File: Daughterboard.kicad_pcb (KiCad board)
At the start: 4 copper layers, 60 parts, among them U1 SI8271GB-IS, U2 SI8271GB-IS, U3 GS61004B, U4 IES0105S09, U5 GS61004B, U6 IES0105S09

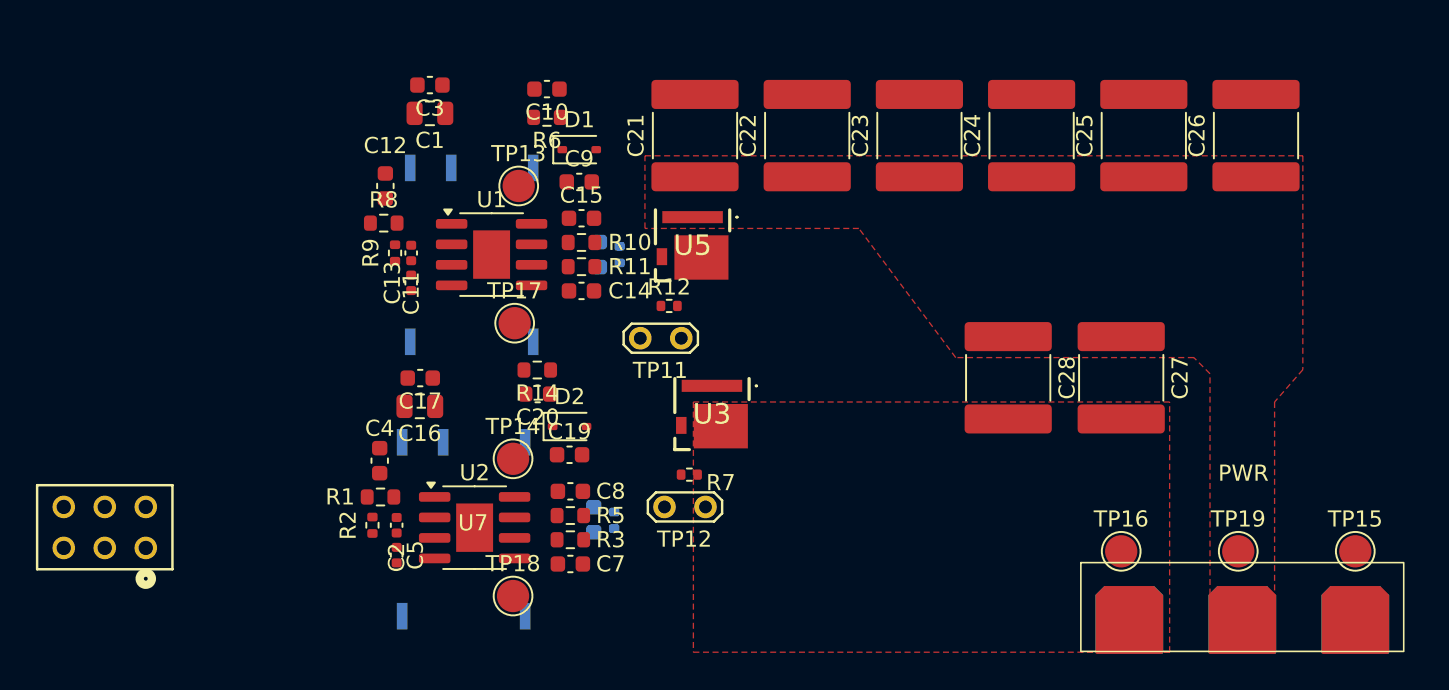
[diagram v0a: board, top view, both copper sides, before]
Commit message: initial version for commenting
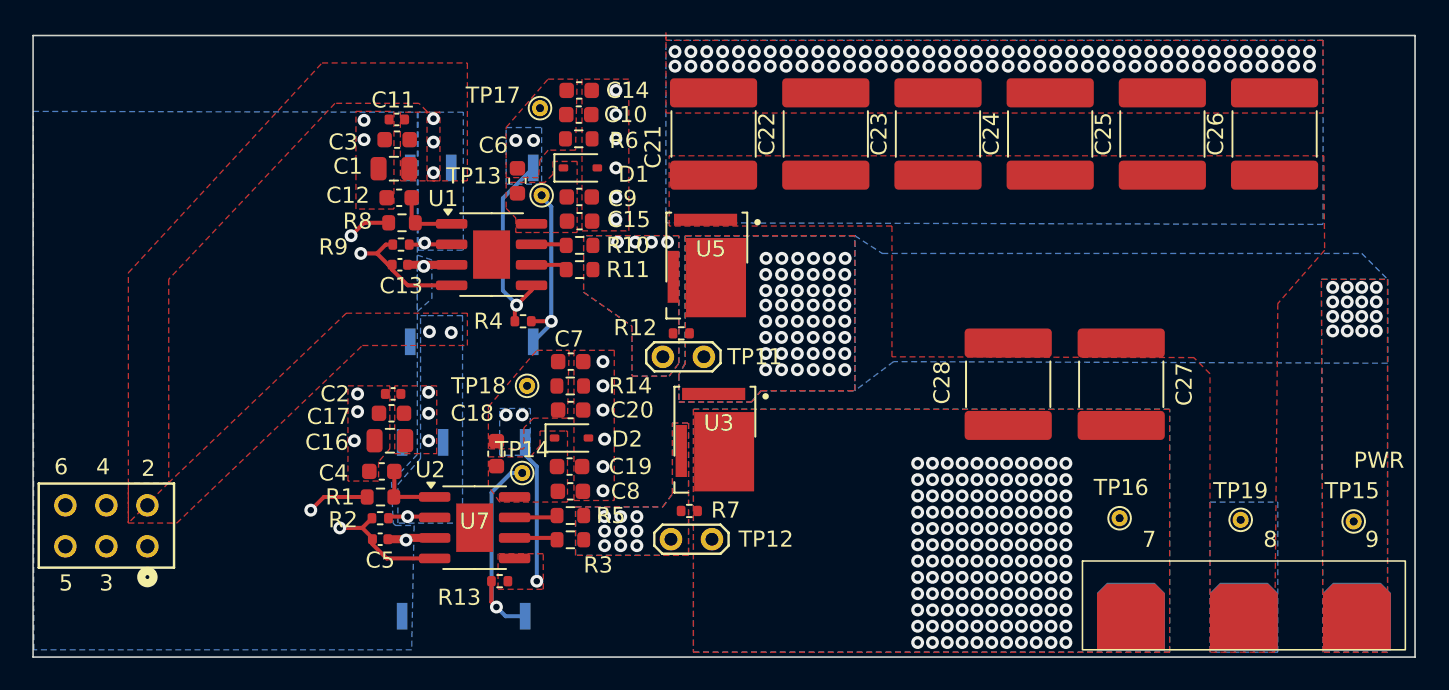
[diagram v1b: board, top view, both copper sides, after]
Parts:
- C18, C6, R13, R4: moved to F.Cu
- TP13, TP14, TP15, TP16, TP17, TP18, TP19: footprint TestPoint:TestPoint_Pad_D2.0mm -> TestPoint:TestPoint_THTPad_D1.0mm_Drill0.5mm
- U3, U5: footprint GS61004B:GS61004B -> GS61004B:GS6XXX4B
- moved TP17 13.4 mm to (110.5, 93.8)
- moved TP18 13.0 mm to (109.7, 111.0)
- moved C7 12.5 mm to (112.4, 109.5)
- moved C14 12.4 mm to (112.9, 92.7)
- moved C11 8.32 mm to (101.6, 94.5), turned to 180 degrees
- moved C2 8.14 mm to (101.4, 111.5), turned to 180 degrees
- moved R13 8.03 mm to (108.0, 123.1), turned to 0 degrees
- moved C18 7.29 mm to (107.8, 115.2)
- moved R4 7.27 mm to (109.5, 107.0), turned to 180 degrees
- moved C6 6.83 mm to (109.1, 98.3)
- moved C1 4.09 mm to (101.5, 97.5)
- moved C3 3.94 mm to (101.7, 95.8)
- moved C16 2.82 mm to (101.2, 114.4)
- moved C17 2.81 mm to (101.3, 112.7)
- moved C10 2.53 mm to (112.9, 94.2)
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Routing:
- net ENABLEH: track 0.00 -> 30.1 mm, vias 0 -> 1
- net PWMH: track 0.00 -> 29.4 mm, vias 0 -> 1
- net PWML: track 0.00 -> 20.8 mm, vias 0 -> 1
- net ENABLEL: track 0.00 -> 20.1 mm, vias 0 -> 1
- net VDDL: track 0.00 -> 13.4 mm, vias 0 -> 1
- net VEEH: track 0.00 -> 12.3 mm, vias 0 -> 3
- net VDDH: track 0.00 -> 11.2 mm, vias 0 -> 1
- net VEEL: track 0.00 -> 8.90 mm, vias 0 -> 3
- net VCC+5V: track 0.00 -> 5.98 mm, vias 0 -> 10
- net GND: track 0.00 -> 5.78 mm, vias 0 -> 7
- net Net-(U2-VI): track 0.00 -> 4.13 mm
- net Net-(U1-VI): track 0.00 -> 3.98 mm
- net DC-: track 0.00 -> 2.74 mm, vias 0 -> 220
- net Net-(U2-VO-): track 0.00 -> 2.68 mm
- net Net-(U2-VO+): track 0.00 -> 2.68 mm
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- added copper zone on B.Cu, net /VgH
- added copper zone on F.Cu, net /VgH
- added copper zone on B.Cu, net /VgL
- added copper zone on F.Cu, net /VgL
- added copper zone on B.Cu, net DC+
- added copper zone on B.Cu, net DC-
- added copper zone on In1.Cu, net DC-
- added copper zone on In2.Cu, net DC-
- added copper zone on B.Cu, net GND
- added copper zone on F.Cu, net GND
- added copper zone on B.Cu, net SW
- added copper zone on F.Cu, net SW
- added copper zone on In1.Cu, net SW
- added copper zone on In2.Cu, net SW
- added copper zone on B.Cu, net VCC+5V
- added copper zone on F.Cu, net VCC+5V
- added copper zone on F.Cu, net VDDH
- added copper zone on F.Cu, net VDDL
- added copper zone on B.Cu, net VEEH
- added copper zone on F.Cu, net VEEH
- added copper zone on B.Cu, net VEEL
- added copper zone on F.Cu, net VEEL
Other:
- board outline added: 85.6 x 38.5 mm
